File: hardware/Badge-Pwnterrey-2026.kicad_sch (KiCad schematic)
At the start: 45 parts, among them J1 Conn_01x08_Socket, J2 Conn_01x08_Socket, J3 Conn_01x10_Socket, J5 Conn_01x10_Socket, P1 USB_C_Plug_USB2.0, Q1 DMP2004TK-7, Q2 DMP2004TK-7, Q3 DMG3415U-7, SW1 RESET, SW2 GPIO, SW3 On, U1 ESP32-C5-WROOM-1-N4, U2 AP2112K-3.3, U3 NT3H2111W0FHK, U4 LNA, U5 GPS

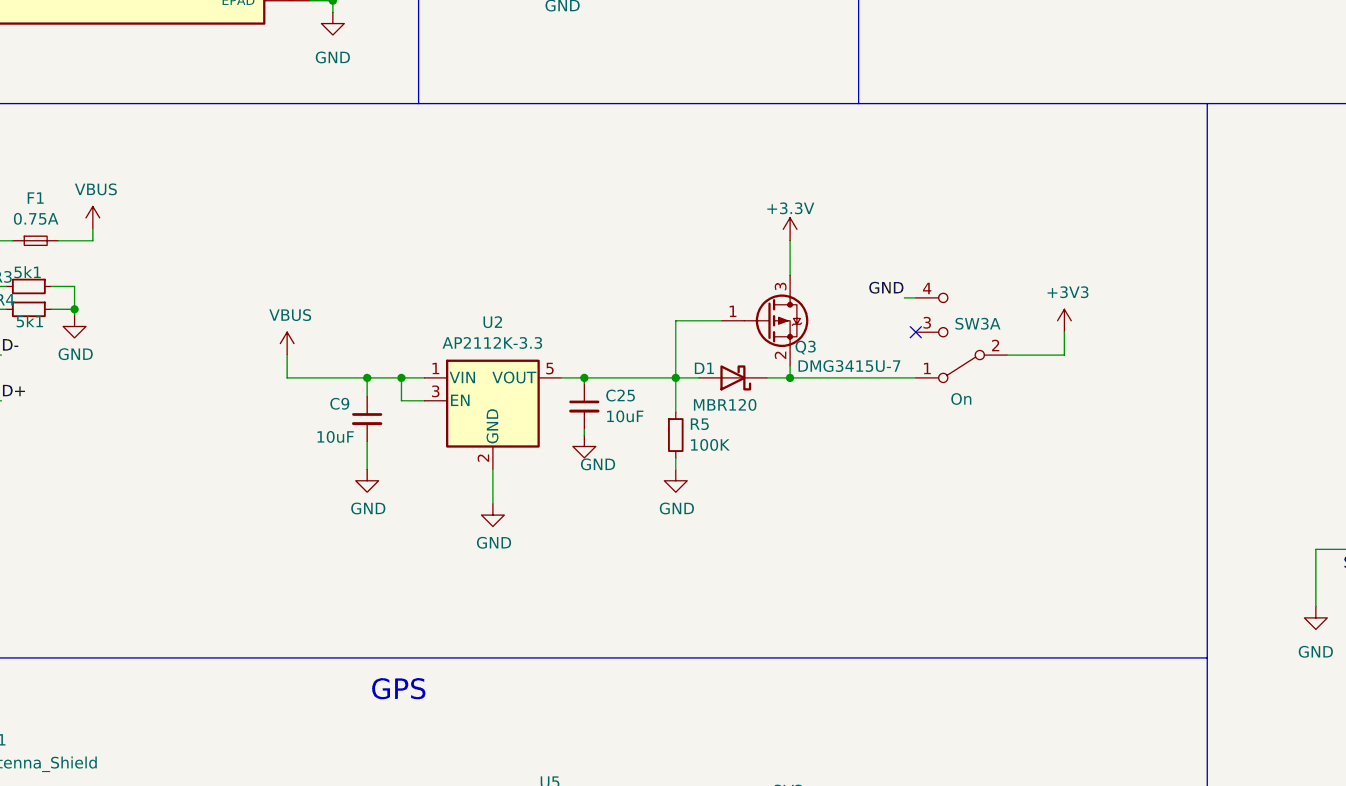
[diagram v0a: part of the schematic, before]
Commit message: feat(hw):Added_TPS2116DRL
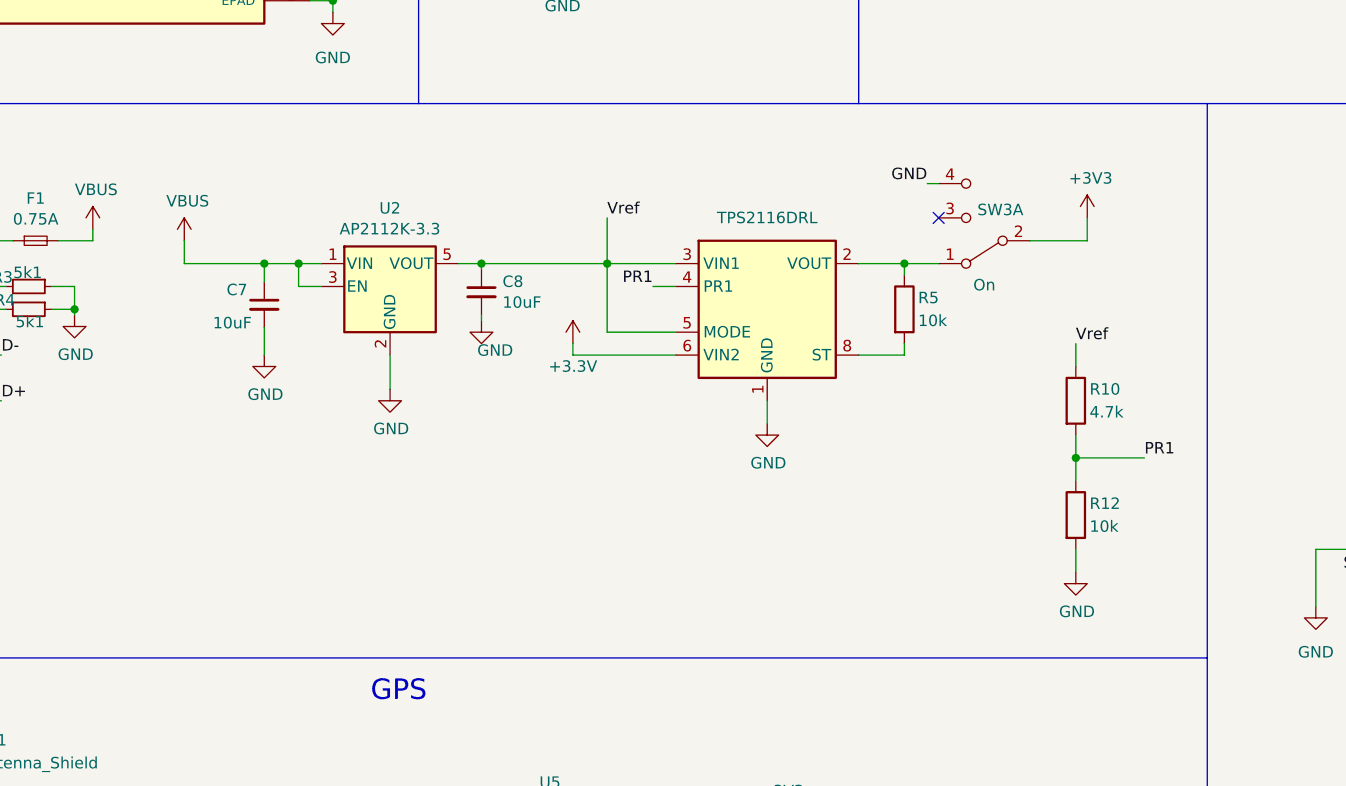
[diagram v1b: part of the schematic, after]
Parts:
- removed C25, C9: 10uF, Capacitor_SMD:C_0603_1608Metric, symbol Device:C_Small
- removed D1: MBR120, Diode_SMD:D_SOD-123F, symbol Diode:MBR340
- removed Q3: DMG3415U-7, Package_TO_SOT_SMD:SOT-23, symbol Device:Q_PMOS_GSD
- removed R5: 100K, Resistor_SMD:R_0603_1608Metric, symbol Device:R_Small
- added C7, C8: 10uF, Capacitor_SMD:C_0603_1608Metric, symbol Device:C_Small
- added R10: 4.7k, Resistor_SMD:R_0603_1608Metric, symbol Device:R
- added R12, R5: 10k, Resistor_SMD:R_0603_1608Metric, symbol Device:R
- added U7: TPS2116DRL, Package_TO_SOT_SMD:SOT-583-8, symbol Power_Management:TPS2116DRL
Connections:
- net +3.3V: now also U7.6 (VIN2)
- net EPAD: now also C7.2, C8.2, R12.2, U7.1 (GND)
- net VBUS: now also C7.1
- net Vref: now reaches U2.5 (VOUT)
- net Vref: now also C8.1, R10.1, U7.3 (VIN1), U7.5 (MODE)
- net at SW3.1 (A): now also R5.1, U7.2 (VOUT), U7.7 (VOUT)
- new net: R5.2, U7.8 (ST)
- new net PR1: R10.2, R12.1, U7.4 (PR1)
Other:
- moved on the sheet: SW3A

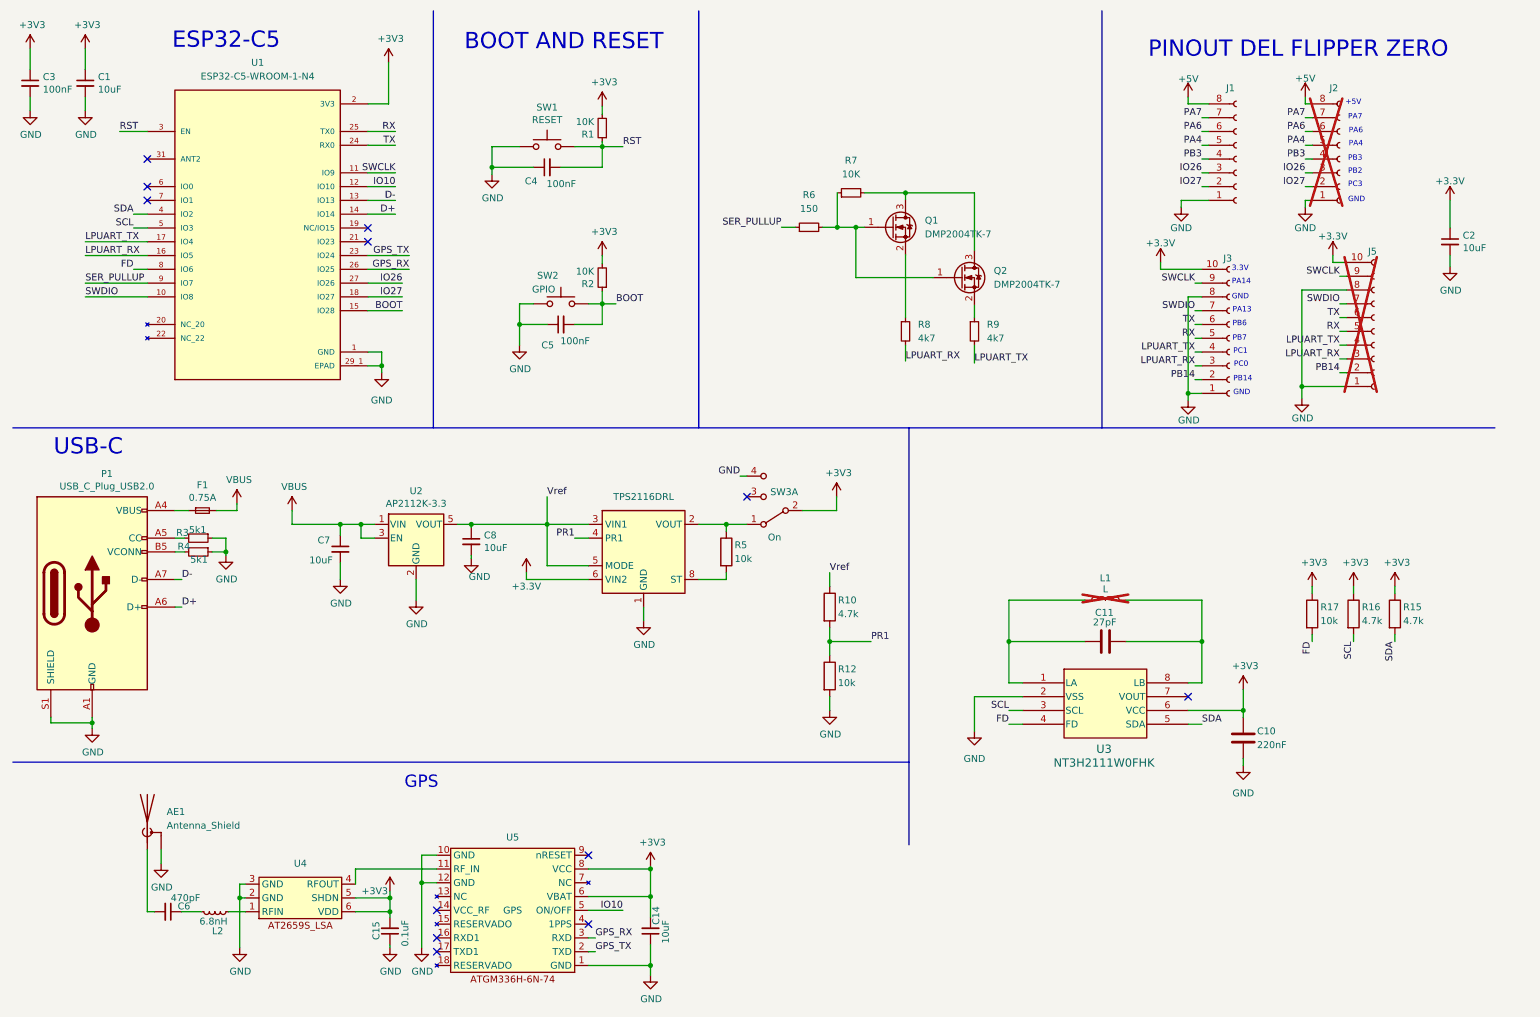
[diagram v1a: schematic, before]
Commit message: feat(Hw):Update_Schematic_And_Route
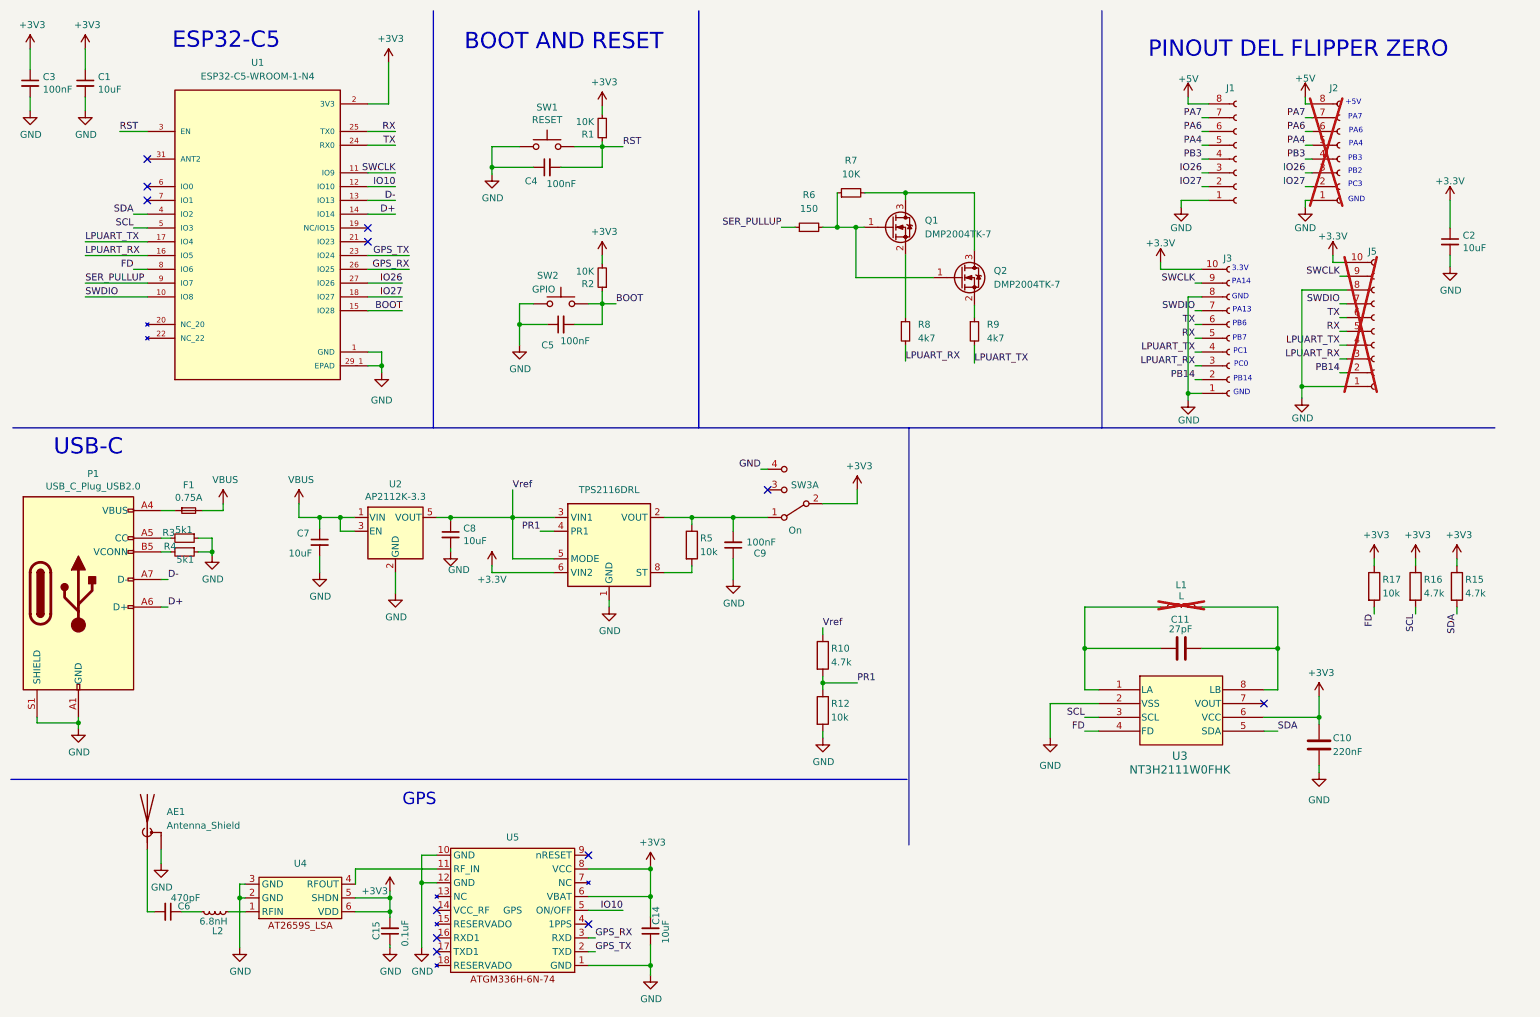
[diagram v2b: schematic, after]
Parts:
- added C9: 100nF, Capacitor_SMD:C_0603_1608Metric, symbol Device:C_Small
- J1, J2: LCSC# C492407 -> C49326132
- J3, J5: LCSC# C57369 -> C49326134
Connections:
- net EPAD: now also C9.1
- net at R5.1, SW3.1 (A), U7.2 (VOUT)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: now also C9.2
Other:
- moved on the sheet: C10, C11, C7, C8, F1, L1, P1, R10, R12, R15, R16, R17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
